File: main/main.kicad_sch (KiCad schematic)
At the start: 26 parts, among them J5 Telegraph key, J6 Conn_01x05_Pin, SW6 RotaryEncoder, U1 STM32F411CEU6, U100 AP1117-33, U4 AT24CS64-SSHM, Y1 32768kHz

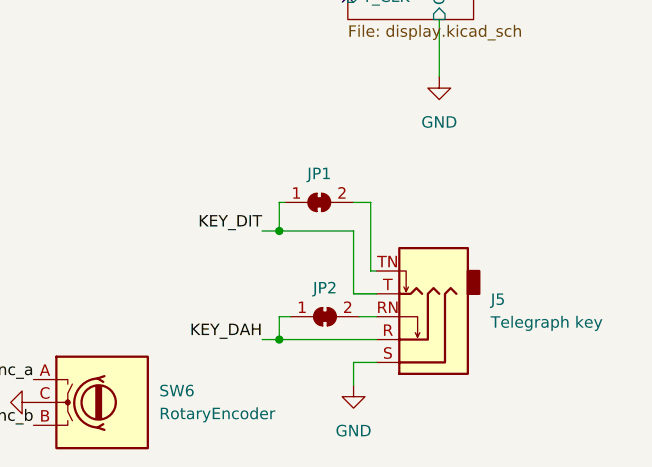
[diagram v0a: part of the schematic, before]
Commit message: Key connector changed, can be used as PTT
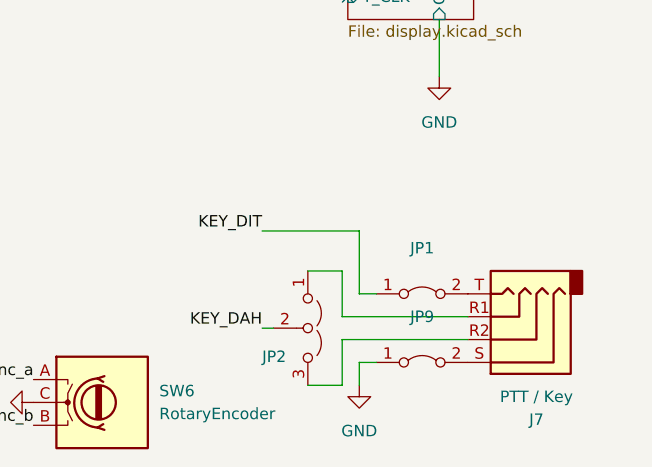
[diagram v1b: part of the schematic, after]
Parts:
- removed J5: Telegraph key, Connector_Audio:Jack_3.5mm_CUI_SJ1-3525N_Horizontal, symbol Connector_Audio:AudioJack3_SwitchTR
- removed JP1, JP2: SolderJumper_2_Bridged, symbol Jumper:SolderJumper_2_Bridged
- added J7: PTT / Key, symbol Connector_Audio:AudioJack4
- added JP1, JP9: Jumper_2_Bridged, symbol Jumper:Jumper_2_Bridged
- added JP2: Jumper_3_Open, symbol Jumper:Jumper_3_Open
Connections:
- net GND: now also JP9.1 (A)
- net KEY_DAH: now also JP2.2 (C)
- net KEY_DIT: now also JP1.1 (A)
- new net: J7.R1, JP2.1 (A)
- new net: J7.R2, JP2.3 (B)
- new net: J7.S, JP9.2 (B)
- new net: J7.T, JP1.2 (B)
